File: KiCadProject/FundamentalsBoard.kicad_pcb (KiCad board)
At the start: 2 copper layers, 62 parts, among them P1 CONN_02X02, P10 CONN_02X02, P11 CONN_01X03, P12 CONN_01X03, P2 CONN_02X02, P3 USB_OTG, P4 CONN_02X02, P5 CONN_01X03, P6 CONN_02X02, P7 CONN_02X02, P8 CONN_02X02, P9 CONN_01X03, Q1 BC550, Q2 BC550, Q3 BC550, U1 MCP601, U2 MCP601, U3 MCP601, U4 MCP601, U5 MCP601, U6 MCP601

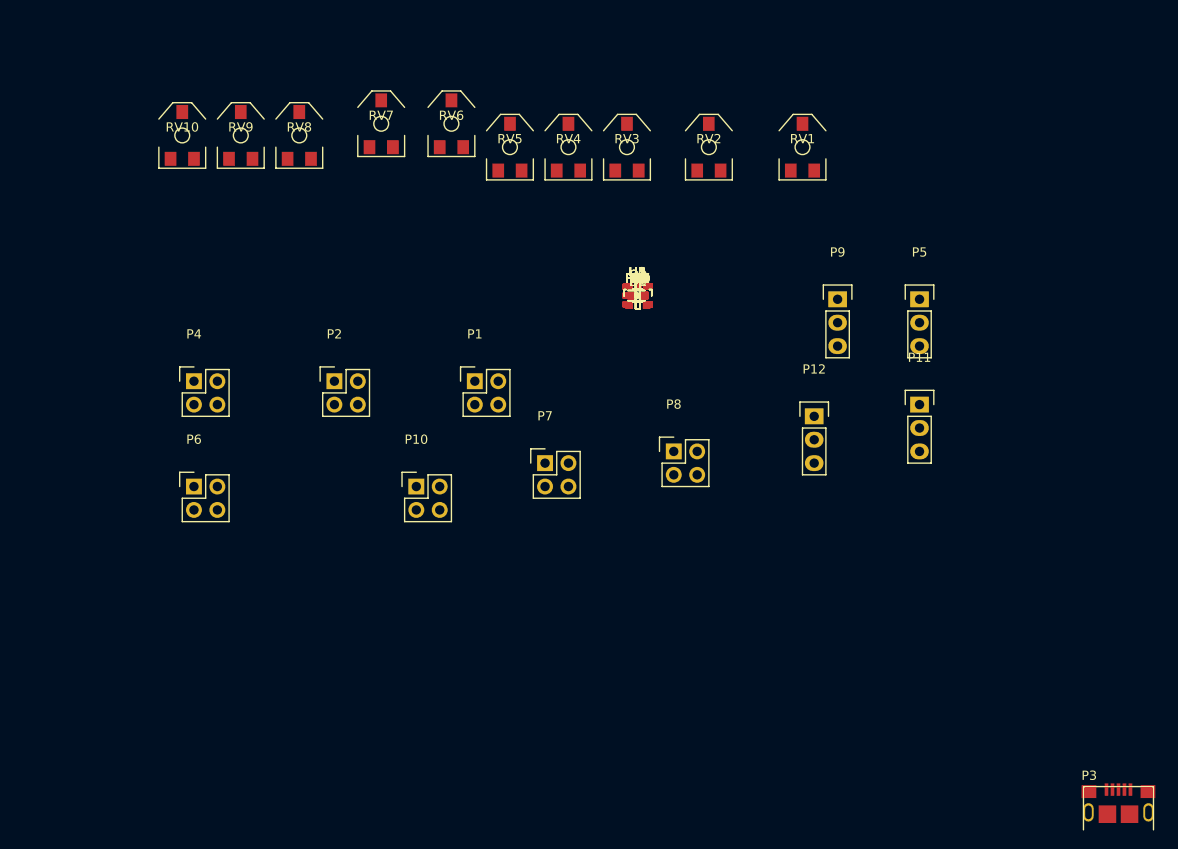
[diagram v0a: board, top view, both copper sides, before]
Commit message: Initial layout
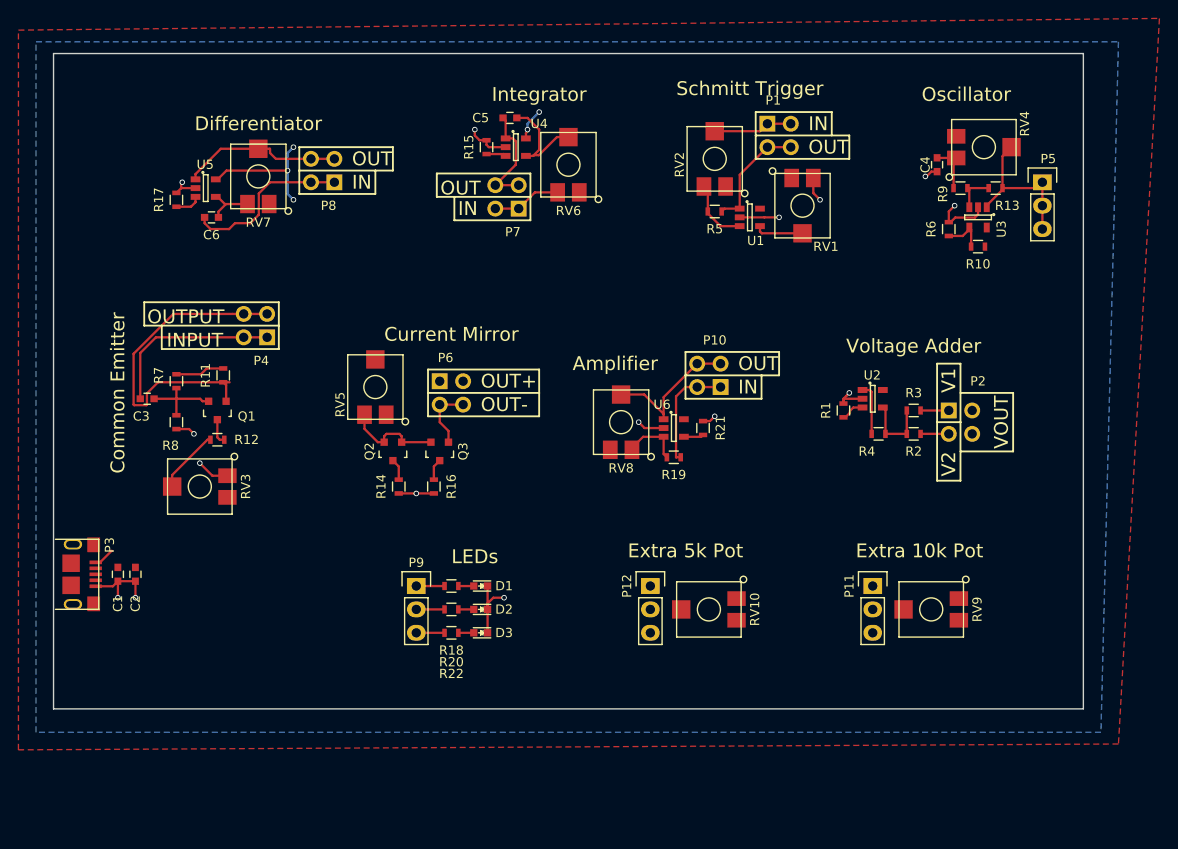
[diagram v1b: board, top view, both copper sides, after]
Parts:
- P1, P10, P2, P4, P6, P7, P8: footprint Pin_Headers:Pin_Header_Straight_2x02 -> TylerCustom:Pin_Header_Straight_2x02
- RV1, RV10, RV2, RV3, RV4, RV5, RV6, RV7, RV8, RV9: footprint SMD_Packages:POT_SMD -> TylerCustom:ST-4
- moved P3 116.6 mm to (83.2, 130.2), turned to 270 degrees
- moved RV9 90.9 mm to (176.5, 134.0), turned to 90 degrees
- moved RV10 76.9 mm to (152.4, 134.0), turned to 90 degrees
- moved P2 66.8 mm to (178.4, 112.4)
- moved C1 64.0 mm to (88.3, 130.2), turned to 90 degrees
- moved C2 62.4 mm to (90.2, 130.2), turned to 90 degrees
- moved RV3 59.2 mm to (97.2, 120.7), turned to 90 degrees
- moved P9 55.3 mm to (120.7, 131.4)
- moved C3 54.4 mm to (91.4, 111.1), turned to 180 degrees
- moved R8 51.9 mm to (94.6, 113.7), turned to 270 degrees
- moved R17 51.1 mm to (94.6, 89.5), turned to 270 degrees
- moved R7 50.9 mm to (94.6, 109.2), turned to 270 degrees
- moved U5 48.3 mm to (97.8, 88.3)
- moved R12 48.2 mm to (99.1, 115.6)
- moved Q1 47.3 mm to (99.1, 112.4), turned to 180 degrees
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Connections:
- C1 pad 2: CMirror_p -> VCC
- C2 pad 2: CMirror_p -> VCC
- P3 pad 1: CMirror_p -> VCC
- P6 pad 1: CMirror_p -> VCC
- P6 pad 2: CMirror_p -> VCC
- R10 pad 1: CMirror_p -> VCC
- R11 pad 1: Net-(R11-Pad1) -> VCC
- R7 pad 1: Net-(R11-Pad1) -> VCC
- RV1 pad 1: CMirror_p -> VCC
- RV5 pad 2: CMirror_p -> VCC
- U1 pad 5: CMirror_p -> VCC
- U2 pad 5: CMirror_p -> VCC
- U3 pad 5: CMirror_p -> VCC
- U4 pad 5: CMirror_p -> VCC
- U5 pad 5: CMirror_p -> VCC
- U6 pad 5: CMirror_p -> VCC
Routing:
- net GND: track 0.00 -> 56.4 mm, vias 0 -> 15
- net C_EmitterOut: track 0.00 -> 36.2 mm
- net VCC: track 0.00 -> 25.5 mm, vias 0 -> 5
- net C_EmitterIn: track 0.00 -> 19.4 mm
- net Diff_in: track 0.00 -> 18.4 mm
- net Diff_out: track 0.00 -> 17.5 mm
- net Net-(P5-Pad1): track 0.00 -> 17.3 mm
- net Amp_out: track 0.00 -> 15.6 mm
- net STrigger_out: track 0.00 -> 12.5 mm
- net Amp_in: track 0.00 -> 12.4 mm
- net Int_out: track 0.00 -> 11.8 mm
- net Net-(C5-Pad1): track 0.00 -> 11.4 mm
- net Net-(Q2-Pad1): track 0.00 -> 10.9 mm
- net Net-(C3-Pad1): track 0.00 -> 8.98 mm
- net STrigger_in: track 0.00 -> 8.59 mm
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- added copper zone on B.Cu, net GND
- added copper zone on F.Cu, net VCC
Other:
- board outline added: 111.8 x 71.1 mm
- board text added: "Amplifier"
- board text added: "Common Emitter"
- board text added: "Current Mirror"
- board text added: "Differentiator"
- board text added: "Extra 10k Pot"
- board text added: "Extra 5k Pot"
- board text added: "IN"
- board text added: "INPUT"
- board text added: "Integrator"
- board text added: "LEDs"
- board text added: "OUT"
- board text added: "OUT+"
- board text added: "OUT-"
- board text added: "OUTPUT"
- board text added: "Oscillator"
- board text added: "Schmitt Trigger"
- board text added: "V1"
- board text added: "V2"
- board text added: "VOUT"
- board text added: "Voltage Adder"
